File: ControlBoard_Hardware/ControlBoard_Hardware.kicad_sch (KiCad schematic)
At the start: 26 parts, among them U2 TSR_1-2450

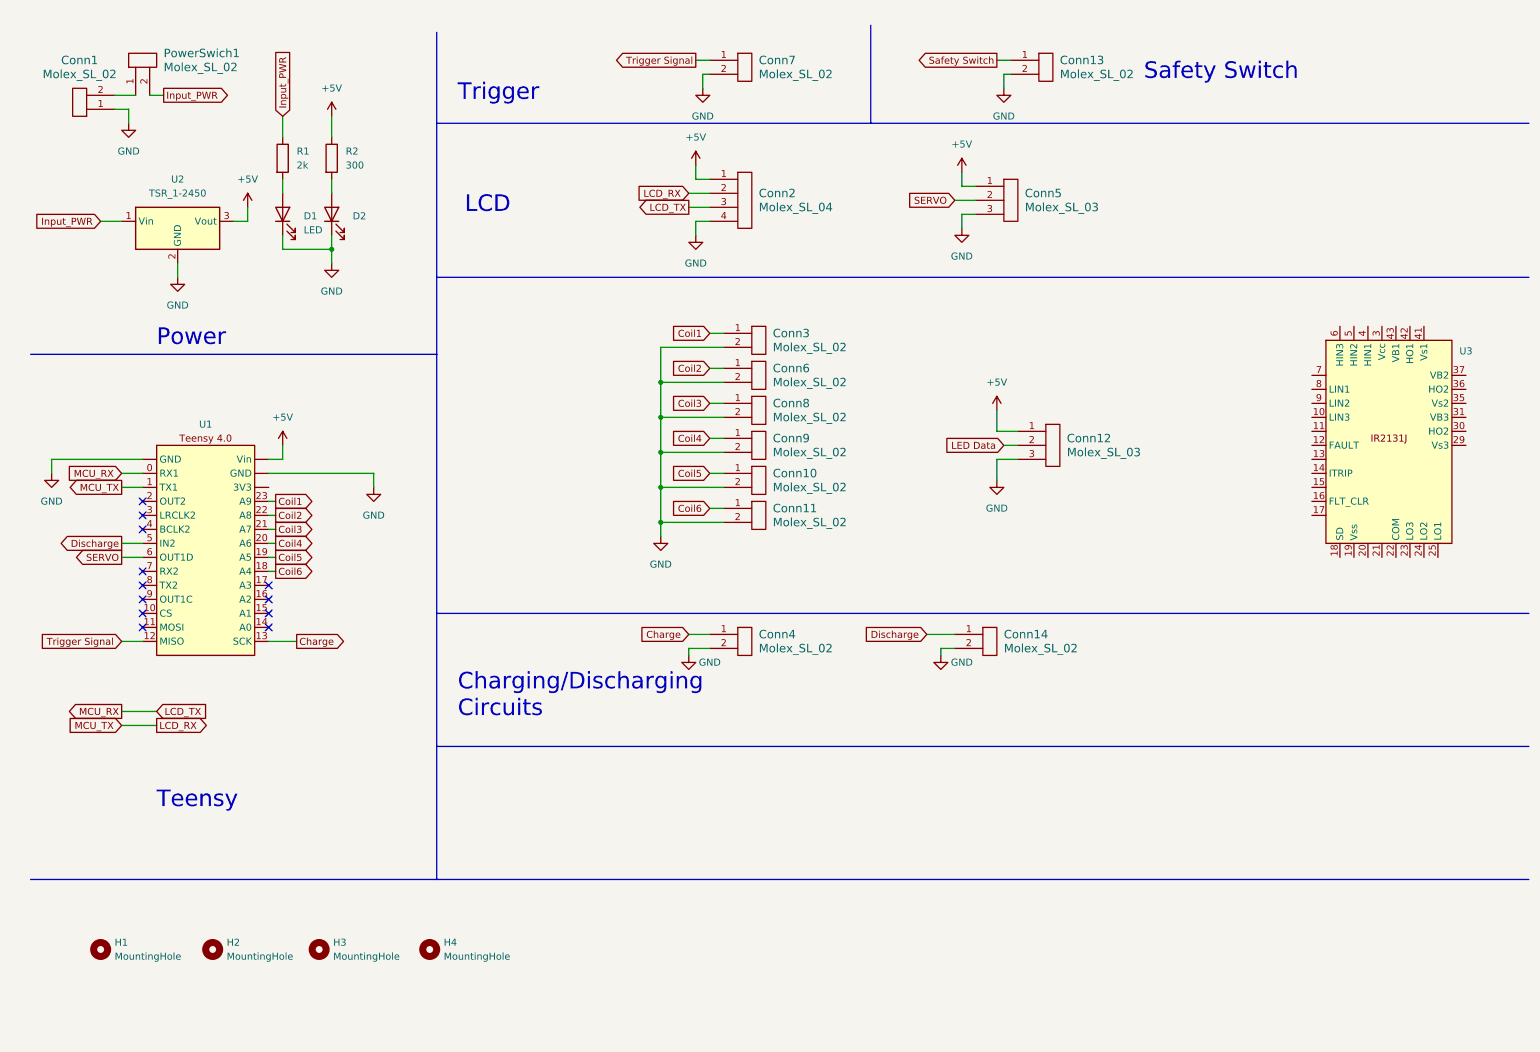
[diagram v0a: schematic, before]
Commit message: updated schematic
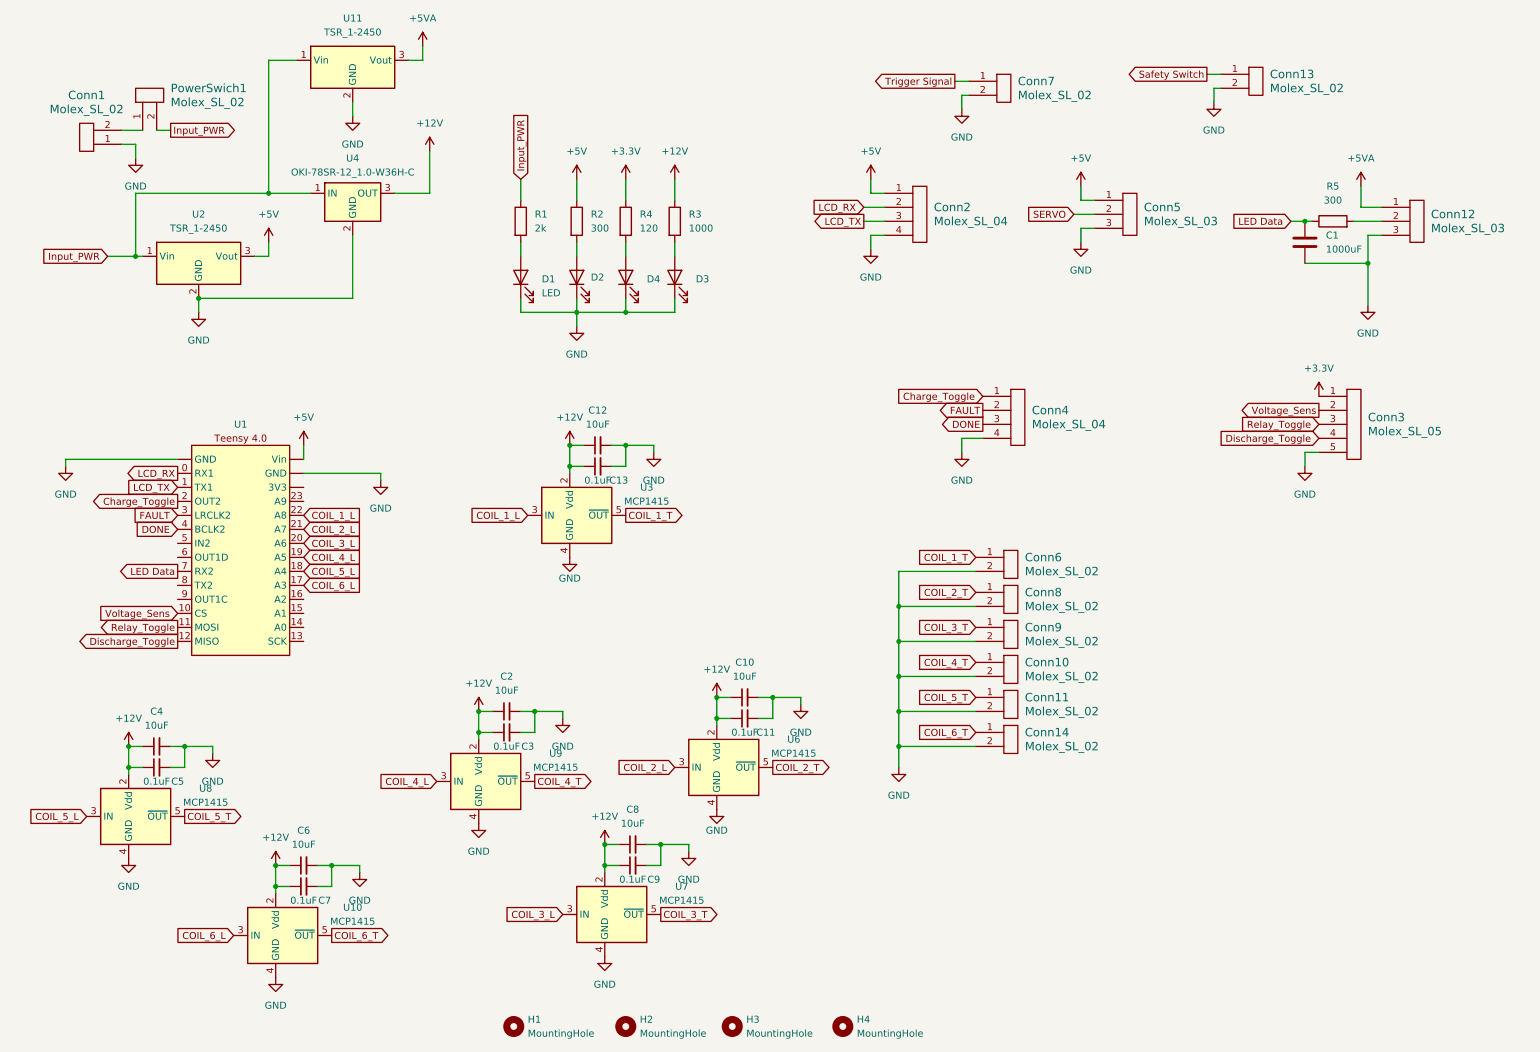
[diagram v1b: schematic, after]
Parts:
- removed Conn3, Conn4: Molex_SL_02, MRDT_Connectors:MOLEX_SL_02_Horizontal, symbol MRDT_Connectors:Molex_SL_02
- removed U3: ~, Package_LCC:PLCC-44_THT-Socket, symbol GateDriver:IR2131J
- added C1: 1000uF, https://www.mouser.com/datasheet/2/447/KEM_A4004_ESK-3316395.pdf, symbol Device:C
- added C10, C12, C2, C4, C6, C8: 10uF, symbol Device:C_Small
- added C11, C13, C3, C5, C7, C9: 0.1uF, symbol Device:C_Small
- added Conn3: Molex_SL_05, symbol MRDT_Connectors:Molex_SL_05
- added Conn4: Molex_SL_04, MRDT_Connectors:MOLEX_SL_04_Horizontal, symbol MRDT_Connectors:Molex_SL_04
- added D3, D4: LED, LED_SMD:LED_0603_1608Metric_Pad1.05x0.95mm_HandSolder, symbol Device:LED
- added R3: 1000, Resistor_SMD:R_0603_1608Metric_Pad0.98x0.95mm_HandSolder, symbol Device:R
- added R4: 120, Resistor_SMD:R_0603_1608Metric_Pad0.98x0.95mm_HandSolder, symbol Device:R
- added R5: 300, symbol Device:R
- added U10, U3, U6, U7, U8, U9: MCP1415, Package_TO_SOT_SMD:SOT-23-5, symbol Driver_FET:MCP1415
- added U11: TSR_1-2450, Converter_DCDC:Converter_DCDC_TRACO_TSR-1_THT, symbol Regulator_Switching:TSR_1-2450
- added U4: OKI-78SR-12_1.0-W36H-C, Converter_DCDC:Converter_DCDC_Murata_OKI-78SR_Horizontal, symbol Converter_DCDC:OKI-78SR-12_1.0-W36H-C
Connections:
- net +5V: no longer Conn12.1
- net GND: now also C1.2, C10.2, C11.2, C12.2, C13.2, C2.2, C3.2, C4.2, C5.2, C6.2, C7.2, C8.2, C9.2, Conn3.5, Conn4.4, D3.1 (K), D4.1 (K), U10.4 (GND), U11.2 (GND), U3.4 (GND), U4.2 (GND), U6.4 (GND), U7.4 (GND), U8.4 (GND), U9.4 (GND)
- net Input_PWR: now also U11.1 (Vin), U4.1 (IN)
- net LCD_RX: now also U1.0 (RX1); no longer U1.1 (TX1)
- net LCD_TX: now also U1.1 (TX1); no longer U1.0 (RX1)
- net LED Data: now also U1.7 (RX2), C1.1, R5.1; no longer Conn12.2
- net SERVO: no longer U1.6 (OUT1D)
- net Trigger Signal: no longer U1.12 (MISO)
- net Voltage_Sens: now reaches U1.10 (CS)
- net Voltage_Sens: now also Conn3.2
- net Relay_Toggle: now reaches U1.11 (MOSI)
- net Relay_Toggle: now also Conn3.3
- net COIL_6_L: now reaches U1.17 (A3)
- net COIL_6_L: now also U10.3 (IN)
- net Charge_Toggle: now reaches U1.2 (OUT2)
- net Charge_Toggle: now also Conn4.1
- net FAULT: now reaches U1.3 (LRCLK2)
- net FAULT: now also Conn4.2
- net DONE: now reaches U1.4 (BCLK2)
- net DONE: now also Conn4.3
- net Charge: no longer names the net of U1.13 (SCK)
- net Coil1: no longer names the net of U1.23 (A9)
- net Coil2 renamed COIL_1_L
- net COIL_1_L: now also U3.3 (IN); no longer Conn6.1
- net Coil3 renamed COIL_2_L
- net COIL_2_L: now also U6.3 (IN); no longer Conn8.1
- net Coil4 renamed COIL_3_L
- net COIL_3_L: now also U7.3 (IN); no longer Conn9.1
- net Coil5 renamed COIL_4_L
- net COIL_4_L: now also U9.3 (IN); no longer Conn10.1
- net Coil6 renamed COIL_5_L
- net COIL_5_L: now also U8.3 (IN); no longer Conn11.1
- net Discharge: no longer names the net of U1.5 (IN2)
- net Discharge: no longer Conn14.1
- new net: D3.2 (A), R3.2
- new net: D4.2 (A), R4.2
- new net: Conn12.2, R5.2
- new net +12V: C10.1, C11.1, C12.1, C13.1, C2.1, C3.1, C4.1, C5.1, C6.1, C7.1, C8.1, C9.1, R3.1, U10.2 (Vdd), U3.2 (Vdd), U4.3 (OUT), U6.2 (Vdd), U7.2 (Vdd), U8.2 (Vdd), U9.2 (Vdd)
- new net +3.3V: Conn3.1, R4.1
- new net +5VA: Conn12.1, U11.3 (Vout)
- new net COIL_1_T: Conn6.1, U3.5 (~{OUT})
- new net COIL_2_T: Conn8.1, U6.5 (~{OUT})
- new net COIL_3_T: Conn9.1, U7.5 (~{OUT})
- new net COIL_4_T: Conn10.1, U9.5 (~{OUT})
- new net COIL_5_T: Conn11.1, U8.5 (~{OUT})
- new net COIL_6_T: Conn14.1, U10.5 (~{OUT})
- new net Discharge_Toggle: Conn3.4, U1.12 (MISO)
- no-connect marks 12 -> 0
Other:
- note removed: "Charging/Discharging Circuits"
- note removed: "LCD"
- note removed: "Power"
- note removed: "Safety Switch"
- note removed: "Teensy"
- note removed: "Trigger"
- moved on the sheet: Conn1, D1, D2, H1, H2, H3, H4, PowerSwich1, R1, R2, U2
